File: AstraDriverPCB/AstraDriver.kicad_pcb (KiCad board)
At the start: 4 copper layers, 102 x 96 mm, 47 parts, among them CN2 JST VH 2 PIN, CN3 JST VH 2 PIN, CN4 JST VH 2 PIN, CN5 JST VH 2 PIN, CN6 JST VH 8 PIN

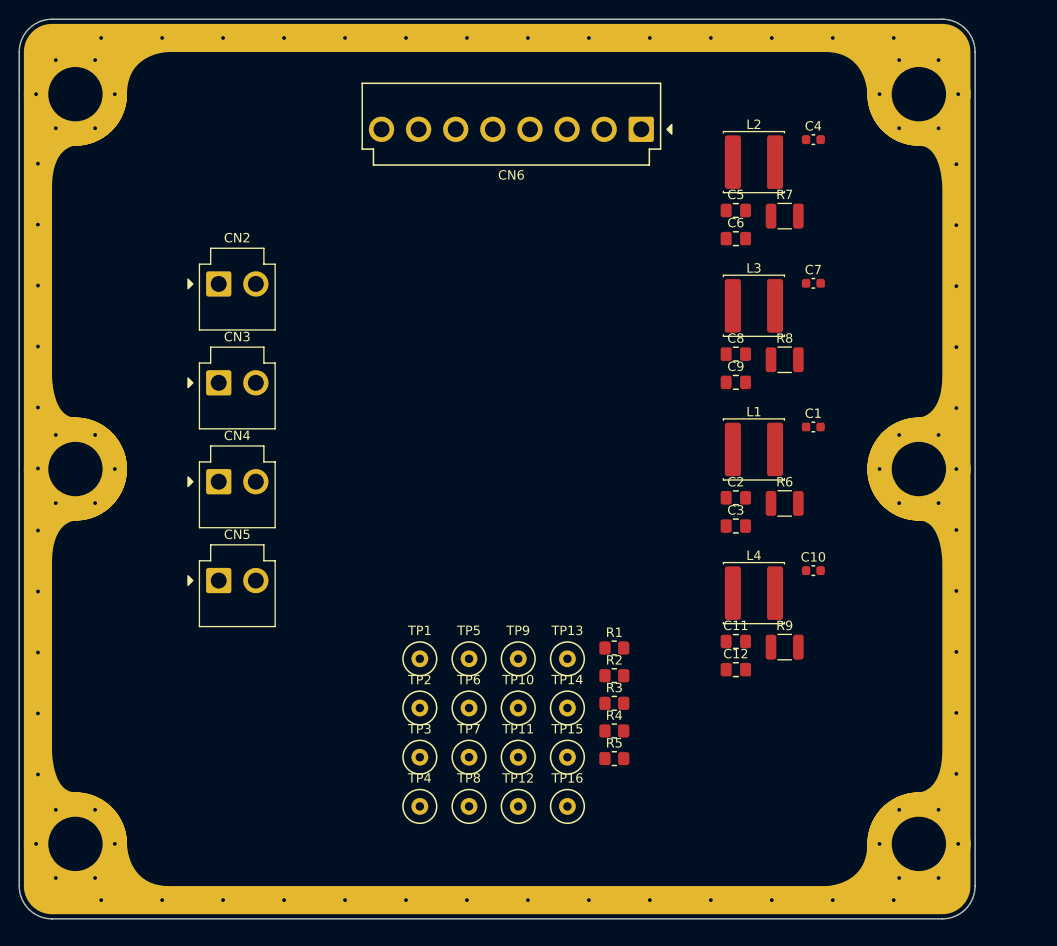
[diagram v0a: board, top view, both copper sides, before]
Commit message: progress
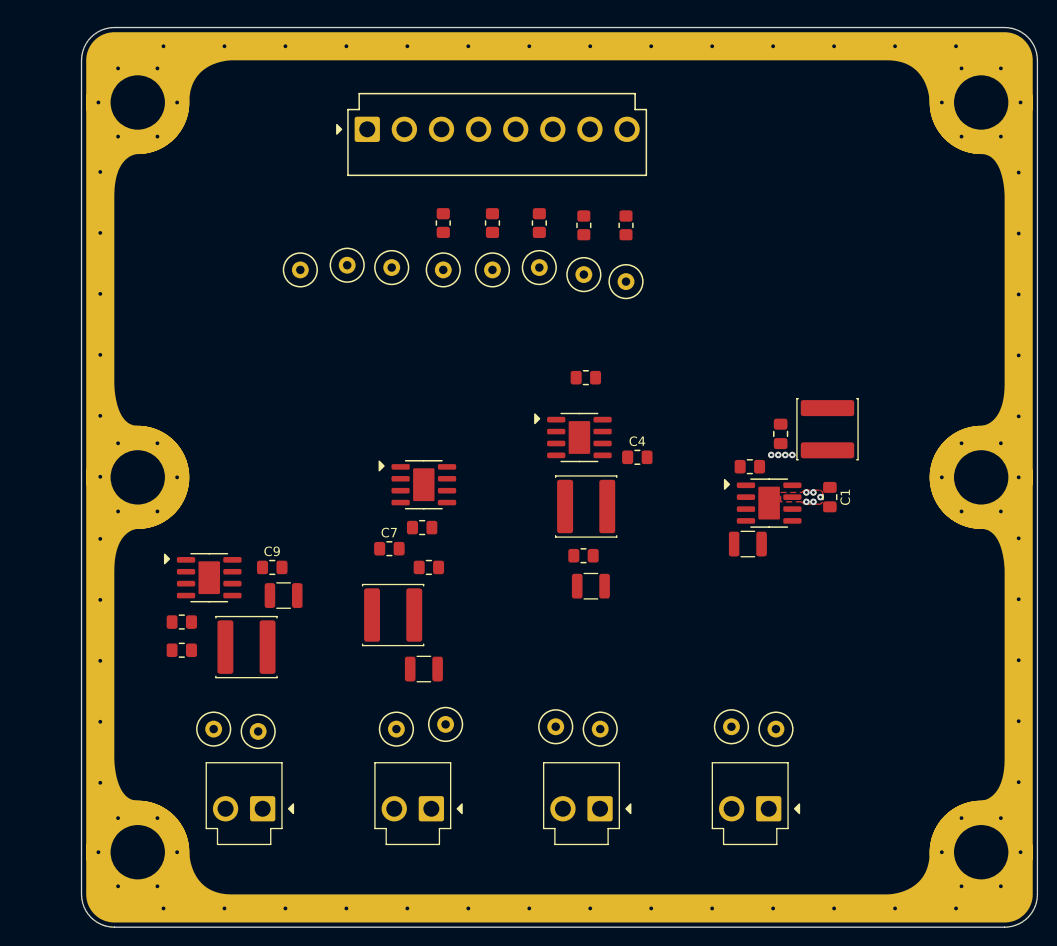
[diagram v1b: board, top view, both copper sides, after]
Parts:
- removed C10: 22u, LiveAstra:C_0603_1608Metric
- removed C11, C12: 1u, LiveAstra:C_0805_2012Metric_Pad1.18x1.45mm_HandSolder
- added C13: 1u, LiveAstra:C_0805_2012Metric_Pad1.18x1.45mm_HandSolder, F.Cu at (178.8, 101.2)
- added C14: 1u, LiveAstra:C_0805_2012Metric_Pad1.18x1.45mm_HandSolder, F.Cu at (157.7, 114.2)
- added C15: 1u, LiveAstra:C_0805_2012Metric_Pad1.18x1.45mm_HandSolder, F.Cu at (141.2, 115.5)
- added U1: LED2001PHR, LiveAstra:U_LED2001PHR_HSOP8, F.Cu at (177.5, 108.6)
- added U2: LED2001PHR, LiveAstra:U_LED2001PHR_HSOP8, F.Cu at (157.3, 101.6)
- added U3: LED2001PHR, LiveAstra:U_LED2001PHR_HSOP8, F.Cu at (140.7, 106.7)
- added U4: LED2001PHR, LiveAstra:U_LED2001PHR_HSOP8, F.Cu at (117.8, 116.6)
- C1, C4, C7: footprint LiveAstra:C_0603_1608Metric -> LiveAstra:C_0805_2012Metric_Pad1.18x1.45mm_HandSolder
- C9: value 1u -> 22u
- moved C6 71.9 mm to (114.8, 121.3)
- moved C8 67.0 mm to (114.8, 124.3)
- moved CN5 59.9 mm to (175.5, 141.2), turned to 180 degrees
- moved TP8 58.5 mm to (162.2, 85.0)
- moved TP4 57.3 mm to (142.8, 83.8)
- moved R5 56.9 mm to (162.2, 79.0), turned to -90 degrees
- moved CN2 56.0 mm to (121.5, 141.2), turned to 180 degrees
- moved L4 54.5 mm to (121.8, 124.0)
- moved R4 54.0 mm to (157.8, 79.0), turned to -90 degrees
- moved R9 53.7 mm to (125.7, 118.5)
- moved C7 53.4 mm to (137.0, 113.5)
- moved C9 53.3 mm to (124.5, 115.5)
- moved TP7 52.9 mm to (157.8, 84.2)
- moved TP3 52.3 mm to (137.2, 83.5)
- moved R3 51.9 mm to (153.0, 78.8), turned to -90 degrees
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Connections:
- net /Block Diagram/Channel 1 2.5A/DIM renamed /Block Diagram/DIM_1
- net /Block Diagram/Channel 1 2.5A/LED- renamed /Block Diagram/CH1_LED-
- net /Block Diagram/Channel 2 2.5A/DIM renamed /Block Diagram/DIM_2
- net /Block Diagram/Channel 3 2.5A/DIM renamed /Block Diagram/DIM_3
- net /Block Diagram/Channel 4 2A/DIM renamed /Block Diagram/DIM_4
- net Net-(R5-Pad2) renamed /Block Diagram/RSRV
- C3 pad 2: /Block Diagram/Channel 1 2.5A/LED+ -> +5V
- C6 pad 2: /Block Diagram/Channel 2 2.5A/LED+ -> /Block Diagram/CH4_LED+
- C9 pad 2: /Block Diagram/Channel 3 2.5A/LED+ -> +5V
- CN2 pad 1: /Block Diagram/Channel 4 2A/LED+ -> /Block Diagram/CH4_LED+
- CN2 pad 2: /Block Diagram/Channel 4 2A/LED- -> /Block Diagram/CH4_LED+
- CN3 pad 1: /Block Diagram/Channel 3 2.5A/LED+ -> /Block Diagram/CH3_LED+
- CN3 pad 2: /Block Diagram/Channel 3 2.5A/LED- -> /Block Diagram/CH3_LED+
- CN4 pad 1: /Block Diagram/Channel 2 2.5A/LED+ -> /Block Diagram/CH2_LED+
- CN4 pad 2: /Block Diagram/Channel 2 2.5A/LED- -> /Block Diagram/CH2_LED+
- CN5 pad 1: /Block Diagram/Channel 1 2.5A/LED+ -> /Block Diagram/CH1_LED+
- CN6 pad 1: /Block Diagram/RESERVED -> +5V
- CN6 pad 2: /Block Diagram/PWM_CH1 -> +3V3
- CN6 pad 3: /Block Diagram/PWM_CH2 -> GND
- CN6 pad 4: /Block Diagram/PWM_CH3 -> /Block Diagram/PWM_CH4
- CN6 pad 5: /Block Diagram/PWM_CH4 -> /Block Diagram/PWM_CH3
- CN6 pad 6: GND -> /Block Diagram/PWM_CH2
- CN6 pad 7: +3V3 -> /Block Diagram/PWM_CH1
- CN6 pad 8: +5V -> /Block Diagram/RESERVED
- L1 pad 1: Net-(U1-SW) -> /Block Diagram/Channel 1 2.5A/SW_OUT
- L1 pad 2: /Block Diagram/Channel 1 2.5A/LED+ -> /Block Diagram/CH1_LED+
- L2 pad 1: Net-(U2-SW) -> /Block Diagram/Channel 2 2.5A/SW_OUT
- L2 pad 2: /Block Diagram/Channel 2 2.5A/LED+ -> /Block Diagram/CH2_LED+
- L3 pad 1: Net-(U3-SW) -> /Block Diagram/Channel 3 2.5A/SW_OUT
- L3 pad 2: /Block Diagram/Channel 3 2.5A/LED+ -> /Block Diagram/CH3_LED+
- L4 pad 1: Net-(U4-SW) -> /Block Diagram/Channel 4 2A/SW_OUT
- L4 pad 2: /Block Diagram/Channel 4 2A/LED+ -> /Block Diagram/CH4_LED+
- R7 pad 2: /Block Diagram/Channel 2 2.5A/LED- -> /Block Diagram/CH2_LED+
- R8 pad 2: /Block Diagram/Channel 3 2.5A/LED- -> /Block Diagram/CH3_LED+
- R9 pad 2: /Block Diagram/Channel 4 2A/LED- -> /Block Diagram/CH4_LED+
- TP10 pad 1: /Block Diagram/Channel 4 2A/LED- -> /Block Diagram/CH4_LED+
- TP11 pad 1: /Block Diagram/Channel 3 2.5A/LED+ -> /Block Diagram/CH3_LED+
- TP12 pad 1: /Block Diagram/Channel 3 2.5A/LED- -> /Block Diagram/CH3_LED+
- TP13 pad 1: /Block Diagram/Channel 2 2.5A/LED+ -> /Block Diagram/CH2_LED+
- TP14 pad 1: /Block Diagram/Channel 2 2.5A/LED- -> /Block Diagram/CH2_LED+
- TP15 pad 1: /Block Diagram/Channel 1 2.5A/LED+ -> /Block Diagram/CH1_LED+
- TP9 pad 1: /Block Diagram/Channel 4 2A/LED+ -> /Block Diagram/CH4_LED+
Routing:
- net GND: vias 0 -> 4
- net /Block Diagram/Channel 1 2.5A/SW_OUT: vias 0 -> 5
- added copper zone on F.Cu, net /Block Diagram/Channel 1 2.5A/SW_OUT
